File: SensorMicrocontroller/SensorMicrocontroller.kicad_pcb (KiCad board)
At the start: 2 copper layers, 100 x 100 mm, 41 parts, among them J1 JST B4B-PH-SM4-TB, J2 JST B4B-PH-SM4-TB, J3 JST B6B-PH-SM4-TB, J4 JST B4B-PH-SM4-TB, J5 JST B4B-PH-SM4-TB, J8 12V Connector, J9 Light Connector, Q1 DMT6009LCT, Q2 DMT6009LCT, U1 ADS1115IDGS, U2 Optoisolators, U3 Optoisolators, U4 Optoisolators, U5 Optoisolators, U6 Optoisolators, U7 Optoisolators, U8 Pico

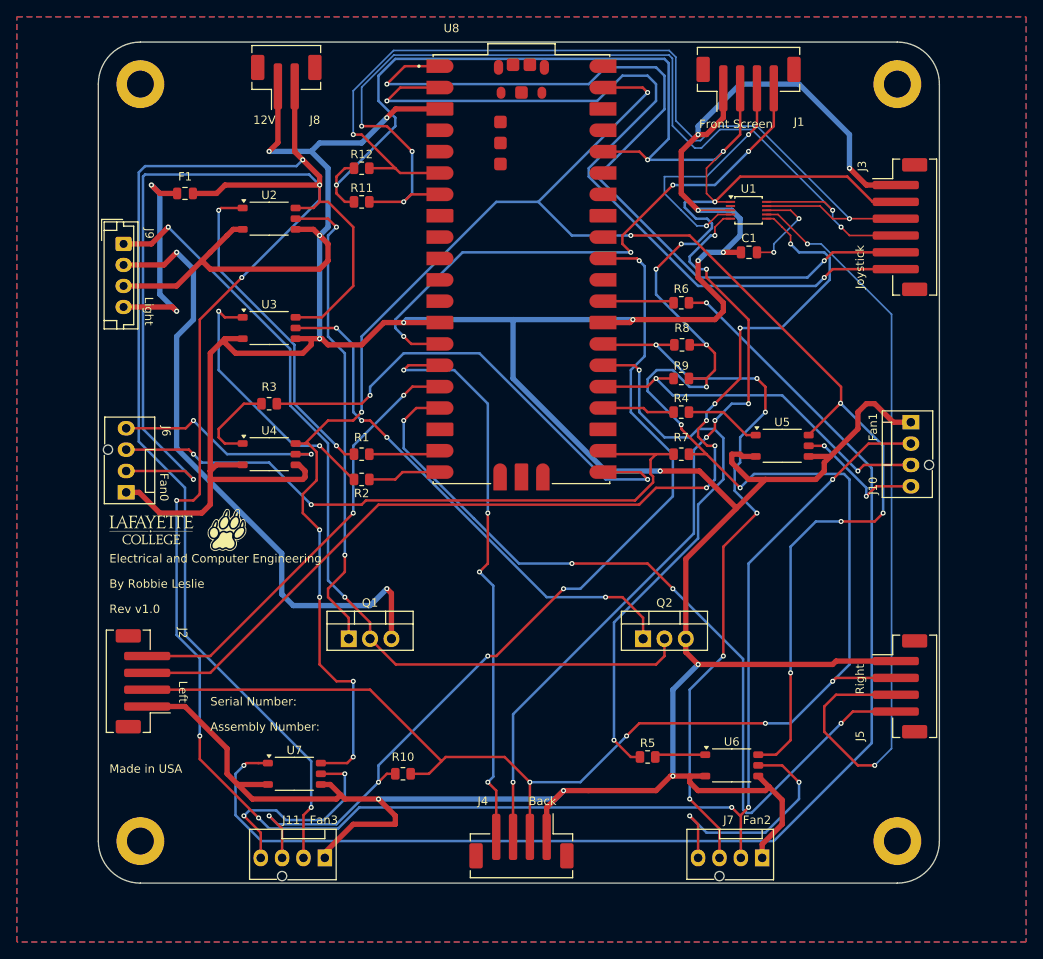
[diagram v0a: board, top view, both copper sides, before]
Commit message: Started re-route
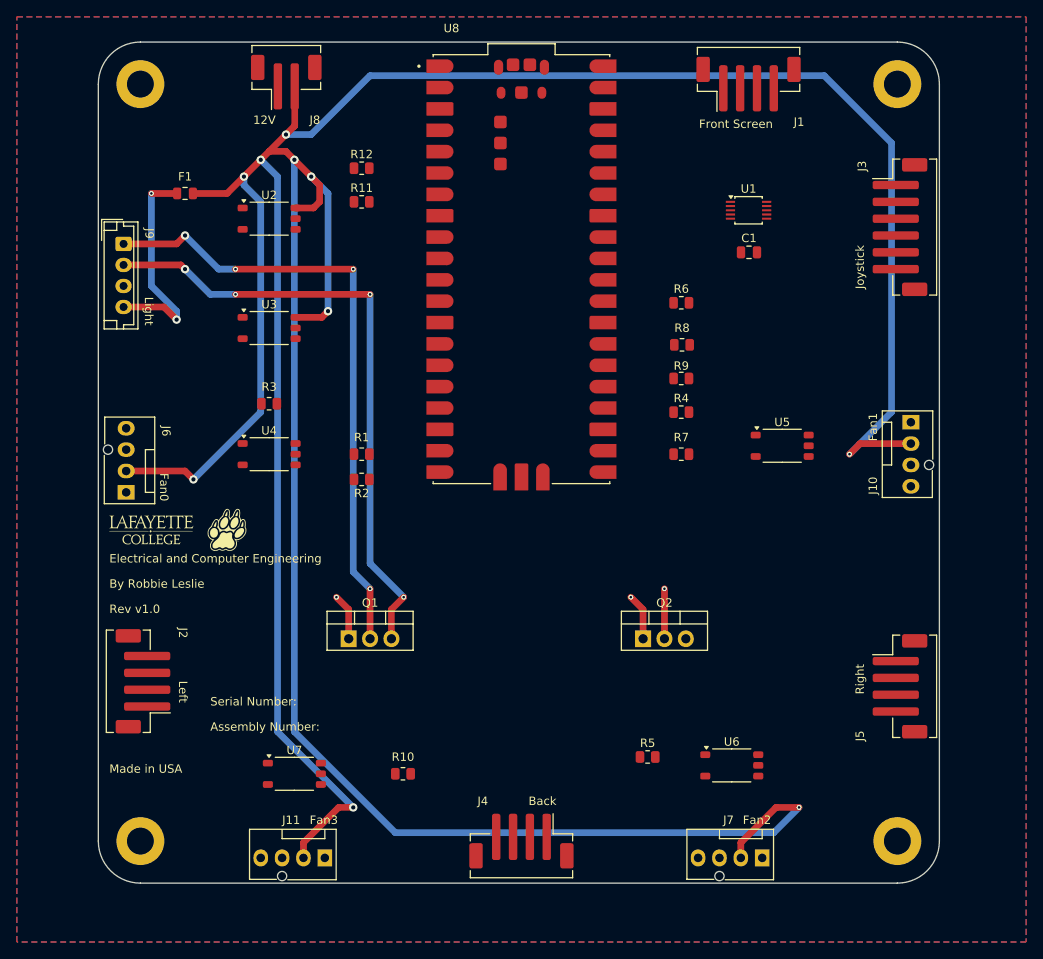
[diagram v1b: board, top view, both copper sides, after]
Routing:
- net /GND: track 560.7 -> 0.00 mm, vias 16 -> 0
- net /3.3V: track 343.7 -> 0.00 mm, vias 14 -> 0
- net /5V: track 224.3 -> 0.00 mm, vias 11 -> 0
- net Net-(U7-Anode): track 153.6 -> 0.00 mm, vias 2 -> 0
- net /US2: track 124.1 -> 0.00 mm, vias 6 -> 0
- net /SCL: track 116.4 -> 0.00 mm, vias 5 -> 0
- net /SDA: track 111.6 -> 0.00 mm, vias 2 -> 0
- net /Fan Sense3: track 109.2 -> 0.00 mm, vias 5 -> 0
- net /PIR3: track 100.2 -> 0.00 mm, vias 4 -> 0
- net /RXFinger: track 98.5 -> 0.00 mm, vias 2 -> 0
- net /TXFinger: track 97.7 -> 0.00 mm, vias 2 -> 0
- net /US3: track 94.0 -> 0.00 mm, vias 2 -> 0
- net /US1: track 92.6 -> 0.00 mm, vias 6 -> 0
- net /Fan Sense2: track 87.0 -> 0.00 mm, vias 6 -> 0
- net /Fan Sense0: track 78.8 -> 0.00 mm, vias 2 -> 0
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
